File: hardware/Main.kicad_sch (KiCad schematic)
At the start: 16 parts, among them SW1 Bourns PEC11R, SW2 Bourns PEC11R, U3 RPi_Pico_TH

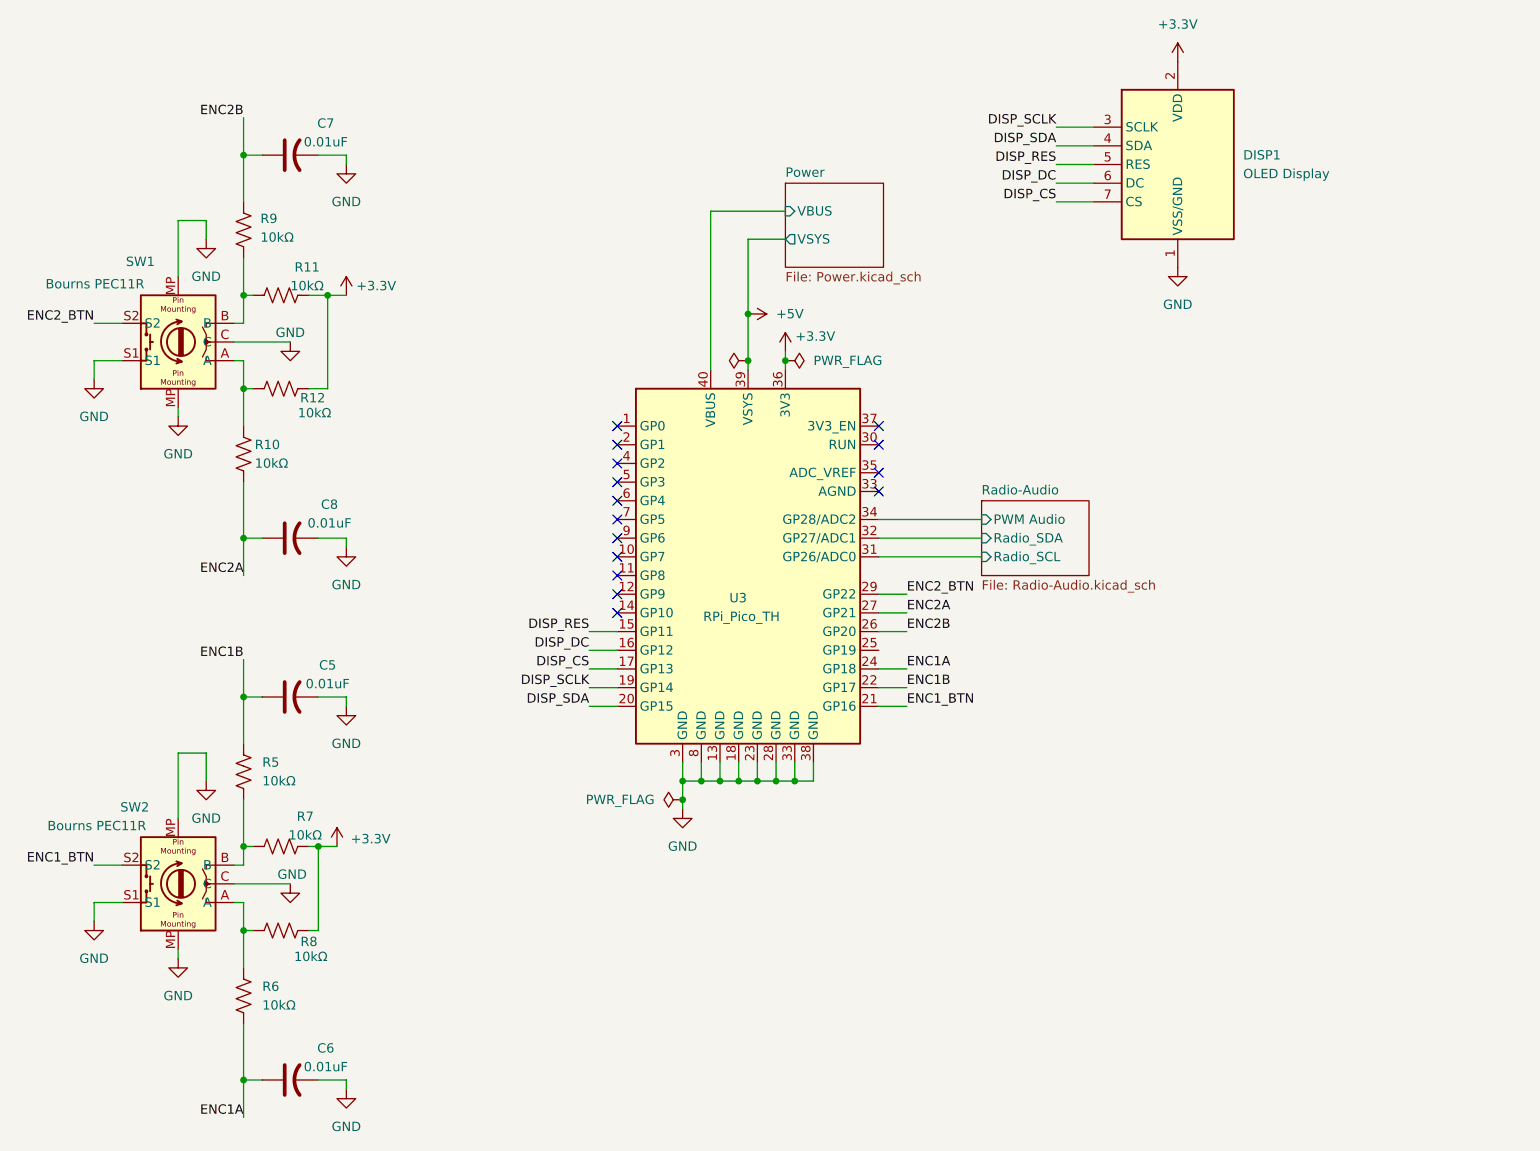
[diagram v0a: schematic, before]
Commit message: Did it all lmao (pcb traces ready for full review)
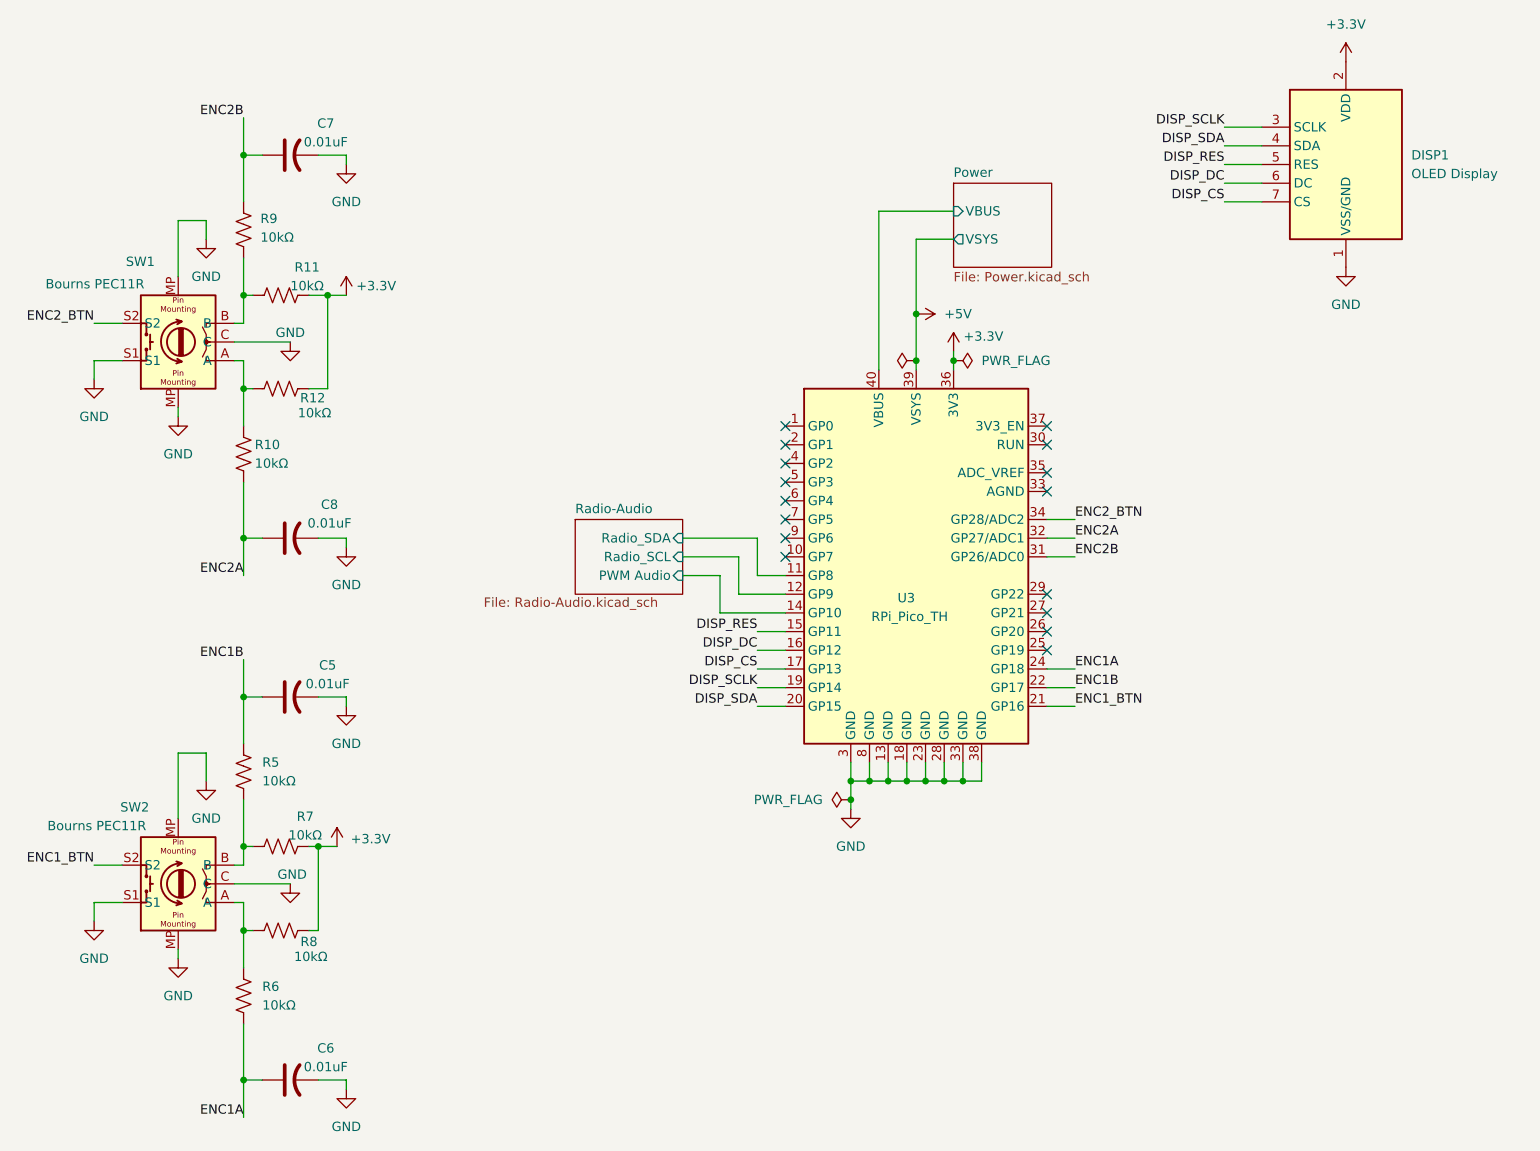
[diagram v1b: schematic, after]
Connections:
- net ENC2A: now also U3.32 (GP27/ADC1); no longer U3.27 (GP21)
- net ENC2B: now also U3.31 (GP26/ADC0); no longer U3.26 (GP20)
- net ENC2_BTN: now also U3.34 (GP28/ADC2); no longer U3.29 (GP22)
- net Radio-Audio/PWM Audio: now also U3.14 (GP10); no longer U3.34 (GP28/ADC2)
- net Radio-Audio/Radio_SCL: now also U3.12 (GP9); no longer U3.31 (GP26/ADC0)
- net Radio-Audio/Radio_SDA: now also U3.11 (GP8); no longer U3.32 (GP27/ADC1)
- no-connect marks 15 -> 16
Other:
- moved on the sheet: DISP1, U3
